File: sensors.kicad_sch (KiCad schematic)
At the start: 20 parts, among them U4 ICM-20602, U5 MMC5983MA, U6 ICP20100

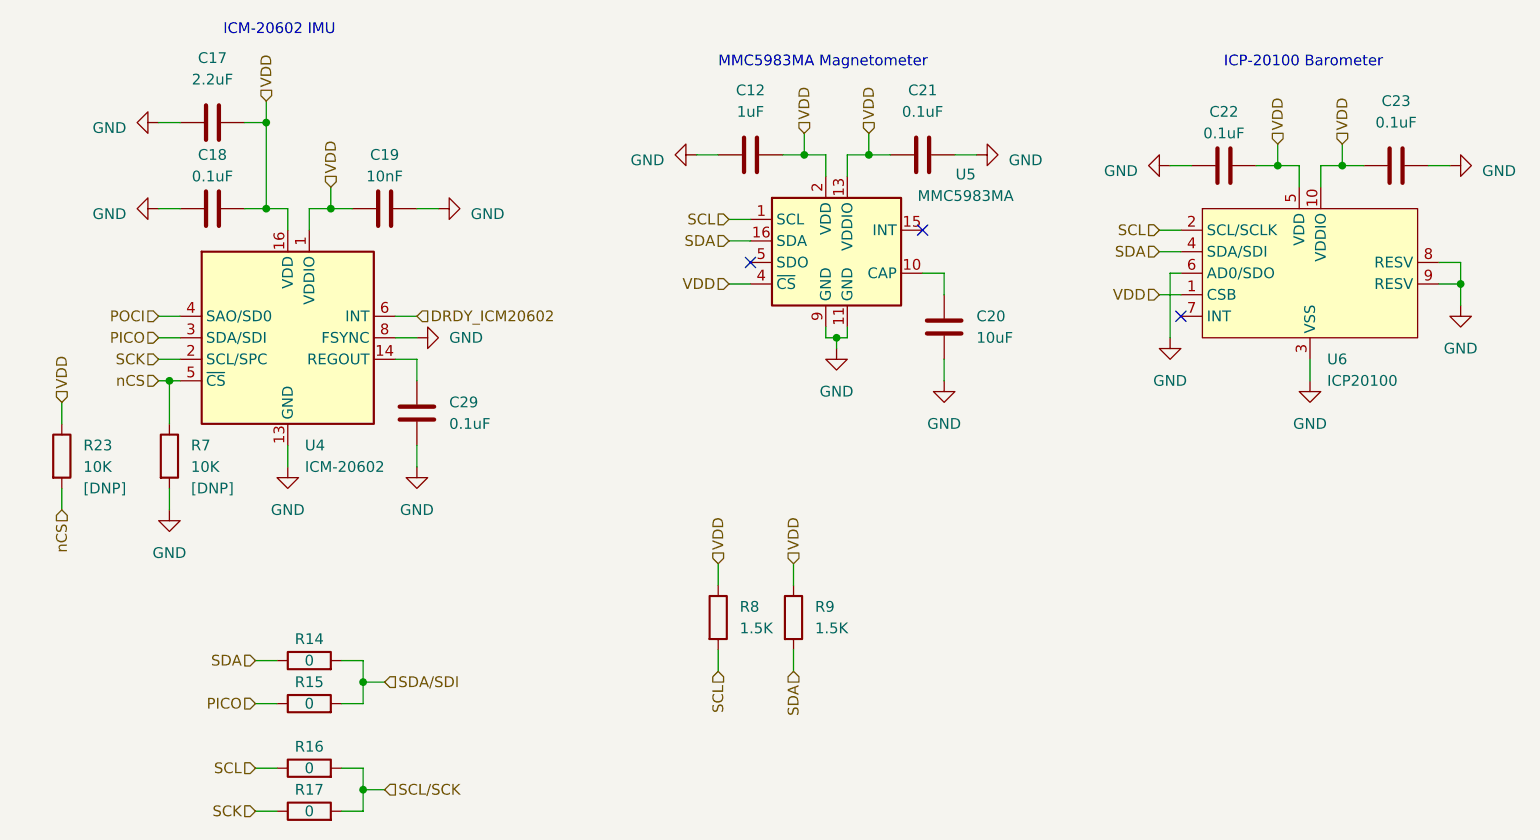
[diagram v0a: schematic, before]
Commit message: R02B: finish new discussion modifications
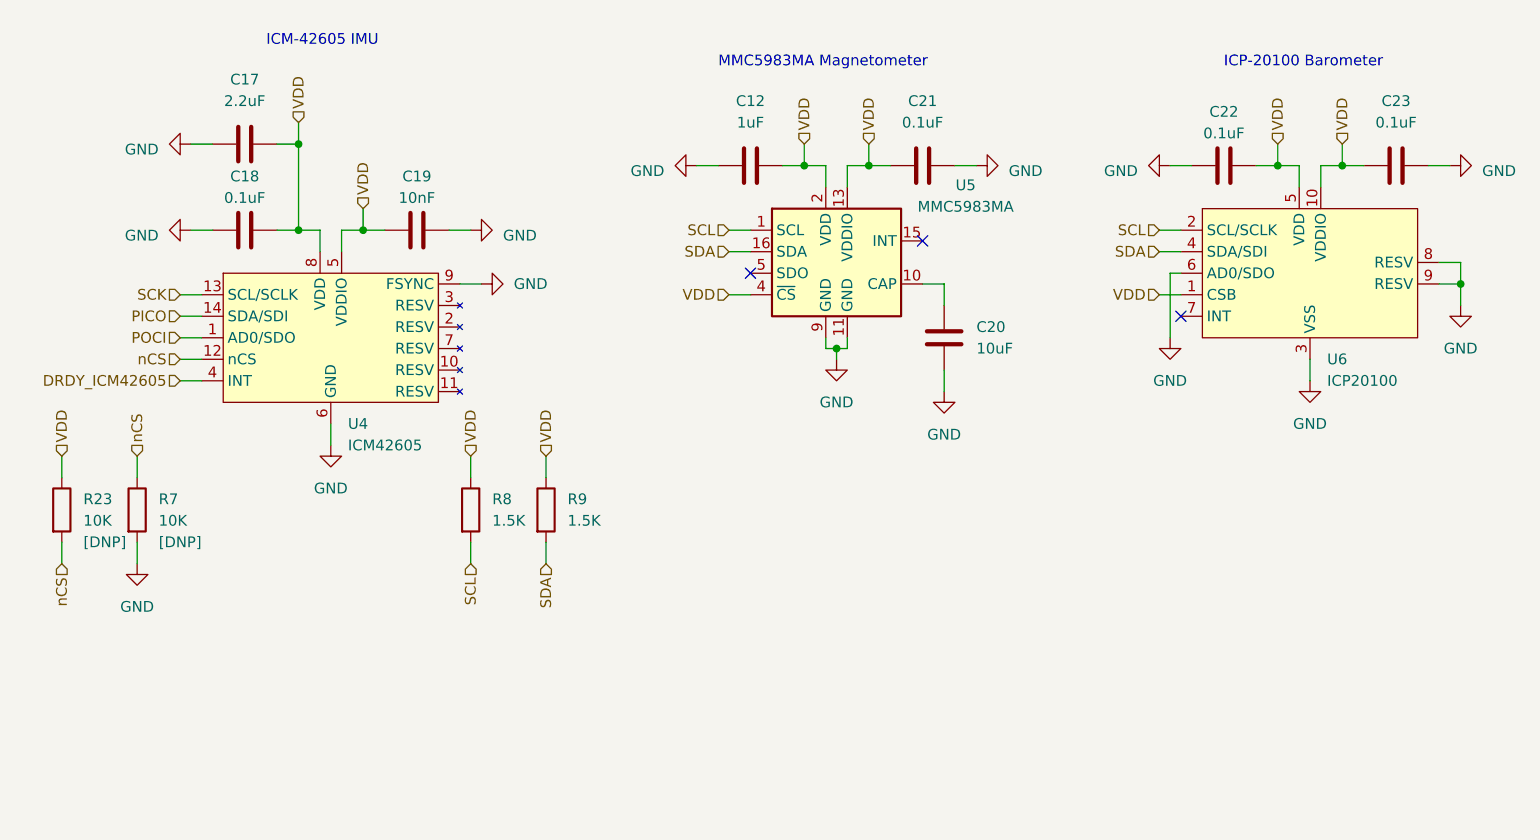
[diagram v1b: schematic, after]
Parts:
- removed C29: 0.1uF, Capacitor_SMD:C_0402_1005Metric, symbol Device:C
- removed R14, R15, R16, R17: 0, Resistor_SMD:R_0402_1005Metric, symbol Device:R
- removed U4: ICM-20602, Package_LGA:LGA-16_3x3mm_P0.5mm_LayoutBorder3x5y, symbol Sensor_Motion:ICM-20602
- added U4: ICM42605, Package_LGA:LGA-14_3x2.5mm_P0.5mm_LayoutBorder3x4y, symbol ICM42605:ICM42605
- C12: footprint Capacitor_SMD:C_0402_1005Metric -> Capacitor_SMD:C_0201_0603Metric
- C17: footprint Capacitor_SMD:C_0402_1005Metric -> Capacitor_SMD:C_0201_0603Metric; Mfr. # (none) -> CC0201MRX5R5BB225
- C18, C21, C22, C23: footprint Capacitor_SMD:C_0402_1005Metric -> Capacitor_SMD:C_0201_0603Metric; Mfr. # (none) -> CC0201KRX5R5BB104
- C19: footprint Capacitor_SMD:C_0402_1005Metric -> Capacitor_SMD:C_0201_0603Metric; Mfr. # (none) -> CC0201KRX5R5BB103
- R8, R9: footprint Resistor_SMD:R_0402_1005Metric -> Resistor_SMD:R_0201_0603Metric
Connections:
- net GND: now also U4.6 (GND), U4.9 (FSYNC)
- net PICO: now also U4.14 (SDA/SDI)
- net POCI: now also U4.1 (AD0/SDO)
- net SCK: now also U4.13 (SCL/SCLK)
- net VDD: now also U4.5 (VDDIO), U4.8 (VDD)
- net nCS: now also U4.12 (nCS)
- new net DRDY_ICM42605: U4.4 (INT)
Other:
- note added: "ICM-42605 IMU"
- note removed: "ICM-20602 IMU"
- moved on the sheet: C12, C17, C18, C19, C20, C21, R23, R7, R8, R9, U5
